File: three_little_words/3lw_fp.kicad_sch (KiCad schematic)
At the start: 19 parts, among them J10 Eurorack_Mono_Jack, J11 Eurorack_Mono_Jack, J12 Eurorack_Mono_Jack, J13 Eurorack_Mono_Jack, J14 Eurorack_Mono_Jack, J2 Eurorack_Mono_Jack, J3 Eurorack_Mono_Jack, J4 Eurorack_Mono_Jack, J5 Eurorack_Mono_Jack, J6 Eurorack_Mono_Jack, J7 Eurorack_Mono_Jack, J8 SSD1306_OLED_CONN, J9 Eurorack_Mono_Jack, SW1 SW_Push, SW2 SW_Push, SW3 SW_Push, SW4 RotaryEncoder_Switch, SW5 RotaryEncoder_Switch, SW6 RotaryEncoder_Switch

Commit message: Adding footprints for various components of 3lw.
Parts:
- J8: footprint (none) -> Connector_PinSocket_2.54mm:PinSocket_1x04_P2.54mm_Vertical
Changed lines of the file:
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@@
     (property "Reference" "J8" (id 0) (at 66.04 170.18 0))
     (property "Value" "SSD1306_OLED_CONN" (id 1) (at 66.04 172.72 0))
-    (property "Footprint" "" (id 2) (at 65.405 180.975 0)
+    (property "Footprint" "Connector_PinSocket_2.54mm:PinSocket_1x04_P2.54mm_Vertical" (id 2) (at 65.405 180.975 0)
       (effects (font (size 1.27 1.27)) hide)
     )

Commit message: Adding BOM, footprints, starting circuit.
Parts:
- J10, J11, J12, J13, J14, J2, J3, J4, J5, J6, J7, J9: footprint winterbloom:WQP-WQP518MA -> winterbloom:WQP518MA
- SW1, SW2, SW3: footprint (none) -> Button_Switch_THT:SW_PUSH_6mm
- SW4, SW5, SW6: footprint (none) -> Rotary_Encoder:RotaryEncoder_Alps_EC12E-Switch_Vertical_H20mm
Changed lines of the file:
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@@
     (property "Reference" "SW4" (id 0) (at 40.6938 111.506 0))
     (property "Value" "RotaryEncoder_Switch" (id 1) (at 40.6938 114.046 0))
-    (property "Footprint" "" (id 2) (at 36.8838 118.364 0)
+    (property "Footprint" "Rotary_Encoder:RotaryEncoder_Alps_EC12E-Switch_Vertical_H20mm" (id 2) (at 36.8838 118.364 0)
       (effects (font (size 1.27 1.27)) hide)
     )
@@
     (property "Reference" "J14" (id 0) (at 65.2048 108.458 0))
     (property "Value" "Eurorack_Mono_Jack" (id 1) (at 65.2048 105.918 0))
-    (property "Footprint" "winterbloom:WQP-WQP518MA" (id 2) (at 65.8398 106.553 0)
+    (property "Footprint" "winterbloom:WQP518MA" (id 2) (at 65.8398 106.553 0)
       (effects (font (size 1.27 1.27)) hide)
     )
@@
     (property "Reference" "SW3" (id 0) (at 40.4398 194.31 0))
     (property "Value" "SW_Push" (id 1) (at 40.4398 191.77 0))
-    (property "Footprint" "" (id 2) (at 40.4398 191.008 0)
+    (property "Footprint" "Button_Switch_THT:SW_PUSH_6mm" (id 2) (at 40.4398 191.008 0)
       (effects (font (size 1.27 1.27)) hide)
     )
@@
     (property "Reference" "J10" (id 0) (at 65.2048 44.958 0))
     (property "Value" "Eurorack_Mono_Jack" (id 1) (at 65.2048 42.418 0))
-    (property "Footprint" "winterbloom:WQP-WQP518MA" (id 2) (at 65.8398 43.053 0)
+    (property "Footprint" "winterbloom:WQP518MA" (id 2) (at 65.8398 43.053 0)
       (effects (font (size 1.27 1.27)) hide)
     )
@@
     (property "Reference" "J13" (id 0) (at 65.2048 92.583 0))
     (property "Value" "Eurorack_Mono_Jack" (id 1) (at 65.2048 90.043 0))
-    (property "Footprint" "winterbloom:WQP-WQP518MA" (id 2) (at 65.8398 90.678 0)
+    (property "Footprint" "winterbloom:WQP518MA" (id 2) (at 65.8398 90.678 0)
       (effects (font (size 1.27 1.27)) hide)
     )
@@
     (property "Reference" "J11" (id 0) (at 65.2048 60.833 0))
     (property "Value" "Eurorack_Mono_Jack" (id 1) (at 65.2048 58.293 0))
-    (property "Footprint" "winterbloom:WQP-WQP518MA" (id 2) (at 65.8398 58.928 0)
+    (property "Footprint" "winterbloom:WQP518MA" (id 2) (at 65.8398 58.928 0)
       (effects (font (size 1.27 1.27)) hide)
     )
@@
     (property "Reference" "J12" (id 0) (at 65.2048 76.708 0))
     (property "Value" "Eurorack_Mono_Jack" (id 1) (at 65.2048 74.168 0))
-    (property "Footprint" "winterbloom:WQP-WQP518MA" (id 2) (at 65.8398 74.803 0)
+    (property "Footprint" "winterbloom:WQP518MA" (id 2) (at 65.8398 74.803 0)
       (effects (font (size 1.27 1.27)) hide)
     )
@@
     (property "Reference" "J2" (id 0) (at 24.0568 15.113 0))
     (property "Value" "Eurorack_Mono_Jack" (id 1) (at 24.0568 17.653 0))
-    (property "Footprint" "winterbloom:WQP-WQP518MA" (id 2) (at 23.4218 17.018 0)
+    (property "Footprint" "winterbloom:WQP518MA" (id 2) (at 23.4218 17.018 0)
       (effects (font (size 1.27 1.27)) hide)
     )
@@
     (property "Reference" "SW2" (id 0) (at 40.386 184.15 0))
     (property "Value" "SW_Push" (id 1) (at 40.386 181.61 0))
-    (property "Footprint" "" (id 2) (at 40.386 180.848 0)
+    (property "Footprint" "Button_Switch_THT:SW_PUSH_6mm" (id 2) (at 40.386 180.848 0)
       (effects (font (size 1.27 1.27)) hide)
     )
@@
     (property "Reference" "SW1" (id 0) (at 40.386 173.99 0))
     (property "Value" "SW_Push" (id 1) (at 40.386 171.45 0))
-    (property "Footprint" "" (id 2) (at 40.386 170.688 0)
+    (property "Footprint" "Button_Switch_THT:SW_PUSH_6mm" (id 2) (at 40.386 170.688 0)
       (effects (font (size 1.27 1.27)) hide)
     )
@@
     (property "Reference" "J3" (id 0) (at 24.0568 30.988 0))
     (property "Value" "Eurorack_Mono_Jack" (id 1) (at 24.0568 33.528 0))
-    (property "Footprint" "winterbloom:WQP-WQP518MA" (id 2) (at 23.4218 32.893 0)
+    (property "Footprint" "winterbloom:WQP518MA" (id 2) (at 23.4218 32.893 0)
       (effects (font (size 1.27 1.27)) hide)
     )
@@
     (property "Reference" "J4" (id 0) (at 24.0568 46.863 0))
     (property "Value" "Eurorack_Mono_Jack" (id 1) (at 24.0568 49.403 0))
-    (property "Footprint" "winterbloom:WQP-WQP518MA" (id 2) (at 23.4218 48.768 0)
+    (property "Footprint" "winterbloom:WQP518MA" (id 2) (at 23.4218 48.768 0)
       (effects (font (size 1.27 1.27)) hide)
     )
@@
     (property "Reference" "J6" (id 0) (at 24.0568 78.613 0))
     (property "Value" "Eurorack_Mono_Jack" (id 1) (at 24.0568 81.153 0))
-    (property "Footprint" "winterbloom:WQP-WQP518MA" (id 2) (at 23.4218 80.518 0)
+    (property "Footprint" "winterbloom:WQP518MA" (id 2) (at 23.4218 80.518 0)
       (effects (font (size 1.27 1.27)) hide)
     )
@@
     (property "Reference" "J5" (id 0) (at 24.0568 62.738 0))
     (property "Value" "Eurorack_Mono_Jack" (id 1) (at 24.0568 65.278 0))
-    (property "Footprint" "winterbloom:WQP-WQP518MA" (id 2) (at 23.4218 64.643 0)
+    (property "Footprint" "winterbloom:WQP518MA" (id 2) (at 23.4218 64.643 0)
       (effects (font (size 1.27 1.27)) hide)
     )
@@
     (property "Reference" "SW5" (id 0) (at 40.6938 128.524 0))
     (property "Value" "RotaryEncoder_Switch" (id 1) (at 40.6938 131.064 0))
-    (property "Footprint" "" (id 2) (at 36.8838 135.382 0)
+    (property "Footprint" "Rotary_Encoder:RotaryEncoder_Alps_EC12E-Switch_Vertical_H20mm" (id 2) (at 36.8838 135.382 0)
       (effects (font (size 1.27 1.27)) hide)
     )
@@
     (property "Reference" "J7" (id 0) (at 24.0568 94.488 0))
     (property "Value" "Eurorack_Mono_Jack" (id 1) (at 24.0568 97.028 0))
-    (property "Footprint" "winterbloom:WQP-WQP518MA" (id 2) (at 23.4218 96.393 0)
+    (property "Footprint" "winterbloom:WQP518MA" (id 2) (at 23.4218 96.393 0)
       (effects (font (size 1.27 1.27)) hide)
     )
@@
     (property "Reference" "SW6" (id 0) (at 40.6938 145.542 0))
     (property "Value" "RotaryEncoder_Switch" (id 1) (at 40.6938 148.082 0))
-    (property "Footprint" "" (id 2) (at 36.8838 152.4 0)
+    (property "Footprint" "Rotary_Encoder:RotaryEncoder_Alps_EC12E-Switch_Vertical_H20mm" (id 2) (at 36.8838 152.4 0)
       (effects (font (size 1.27 1.27)) hide)
     )
@@
     (property "Reference" "J9" (id 0) (at 65.2048 29.083 0))
     (property "Value" "Eurorack_Mono_Jack" (id 1) (at 65.2048 26.543 0))
-    (property "Footprint" "winterbloom:WQP-WQP518MA" (id 2) (at 65.8398 27.178 0)
-      (effects (font (size 1.27 1.27)) hide)
-    )
+    (property "Footprint" "winterbloom:WQP518MA" (id 2) (at 65.8398 27.178 0)
+      (effects (font (size 1.27 1.27)) hide)
+    )

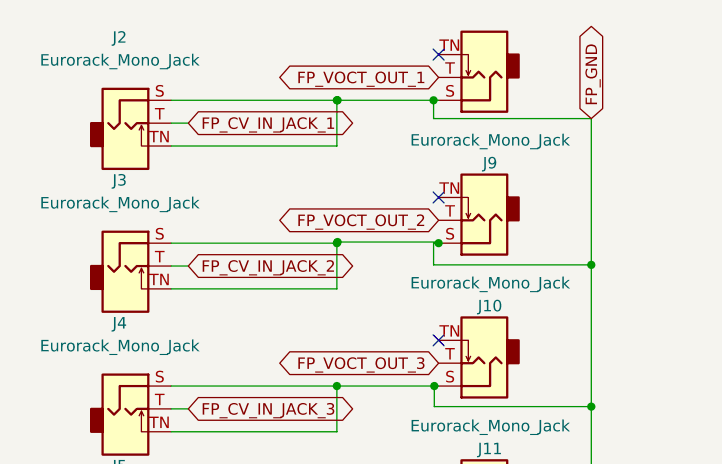
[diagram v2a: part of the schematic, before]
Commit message: Finishing 3lw schematic
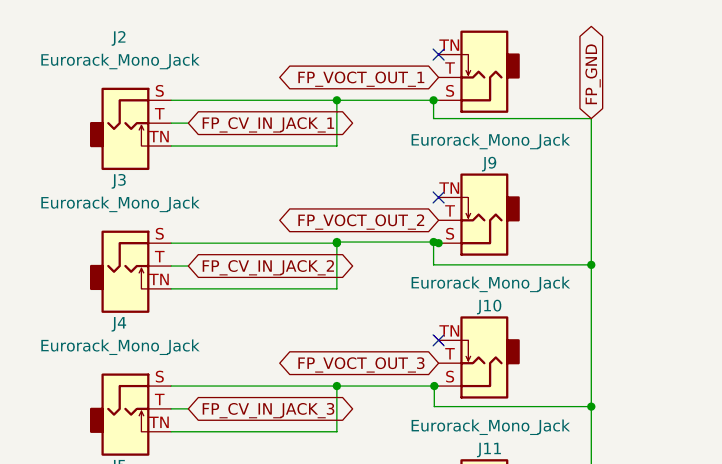
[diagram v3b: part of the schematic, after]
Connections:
- net FP_GND: now also J2.S (Sleeve), J2.TN (Tip_normalize), J3.S (Sleeve), J3.TN (Tip_normalize)
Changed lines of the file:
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@@
   (junction (at 50.0918 101.473) (diameter 0) (color 0 0 0 0)
   )
+  (junction (at 48.1868 37.973) (diameter 0) (color 0 0 0 0)
+  )
+  (junction (at 59.4898 37.973) (diameter 0) (color 0 0 0 0)
+  )
   (junction (at 58.8548 101.473) (diameter 0) (color 0 0 0 0)
   )
+  (junction (at 58.928 22.098) (diameter 0) (color 0 0 0 0)
+  )
+  (junction (at 52.9685 141.986) (diameter 0) (color 0 0 0 0)
+  )
+  (junction (at 76.454 103.886) (diameter 0) (color 0 0 0 0)
+  )
+  (junction (at 76.454 40.386) (diameter 0) (color 0 0 0 0)
+  )
+  (junction (at 48.4313 162.814) (diameter 0) (color 0 0 0 0)
+  )
+  (junction (at 52.3879 159.004) (diameter 0) (color 0 0 0 0)
+  )
+  (junction (at 48.1868 53.848) (diameter 0) (color 0 0 0 0)
+  )
+  (junction (at 58.928 37.846) (diameter 0) (color 0 0 0 0)
+  )
+  (junction (at 59.01 53.848) (diameter 0) (color 0 0 0 0)
+  )
+  (junction (at 76.454 141.986) (diameter 0) (color 0 0 0 0)
+  )
+  (junction (at 76.454 71.882) (diameter 0) (color 0 0 0 0)
+  )
+  (junction (at 50.0918 69.723) (diameter 0) (color 0 0 0 0)
+  )
+  (junction (at 58.8847 85.598) (diameter 0) (color 0 0 0 0)
+  )
   (junction (at 48.1868 22.098) (diameter 0) (color 0 0 0 0)
   )
-  (junction (at 48.1868 37.973) (diameter 0) (color 0 0 0 0)
-  )
-  (junction (at 52.9685 141.986) (diameter 0) (color 0 0 0 0)
-  )
-  (junction (at 48.26 37.846) (diameter 0) (color 0 0 0 0)
-  )
-  (junction (at 76.454 103.886) (diameter 0) (color 0 0 0 0)
-  )
-  (junction (at 76.454 40.386) (diameter 0) (color 0 0 0 0)
-  )
-  (junction (at 48.4313 162.814) (diameter 0) (color 0 0 0 0)
-  )
-  (junction (at 52.3879 159.004) (diameter 0) (color 0 0 0 0)
-  )
-  (junction (at 48.1868 53.848) (diameter 0) (color 0 0 0 0)
-  )
-  (junction (at 59.01 53.848) (diameter 0) (color 0 0 0 0)
-  )
-  (junction (at 76.454 141.986) (diameter 0) (color 0 0 0 0)
-  )
-  (junction (at 58.928 22.098) (diameter 0) (color 0 0 0 0)
-  )
-  (junction (at 76.454 71.882) (diameter 0) (color 0 0 0 0)
-  )
-  (junction (at 50.0918 69.723) (diameter 0) (color 0 0 0 0)
-  )
-  (junction (at 58.8847 85.598) (diameter 0) (color 0 0 0 0)
-  )
   (junction (at 52.6202 124.968) (diameter 0) (color 0 0 0 0)
   )
@@
   (junction (at 76.454 87.884) (diameter 0) (color 0 0 0 0)
   )
-  (junction (at 59.4898 37.973) (diameter 0) (color 0 0 0 0)
-  )
-  (junction (at 48.26 22.098) (diameter 0) (color 0 0 0 0)
-  )
   (junction (at 76.454 124.968) (diameter 0) (color 0 0 0 0)
+  )
+  (junction (at 48.1868 37.846) (diameter 0) (color 0 0 0 0)
   )
   (no_connect (at 59.4898 48.768))
@@
     (stroke (width 0) (type default) (color 0 0 0 0))
   )
+  (wire (pts (xy 59.4898 37.973) (xy 59.4898 37.846))
+    (stroke (width 0) (type default) (color 0 0 0 0))
+  )
   (wire (pts (xy 48.3138 159.004) (xy 52.3879 159.004))
     (stroke (width 0) (type default) (color 0 0 0 0))
   )
-  (wire (pts (xy 58.928 37.973) (xy 59.4898 37.973))
-    (stroke (width 0) (type default) (color 0 0 0 0))
-  )
   (wire (pts (xy 48.1868 53.848) (xy 59.01 53.848))
     (stroke (width 0) (type default) (color 0 0 0 0))
@@
     (stroke (width 0) (type default) (color 0 0 0 0))
   )
+  (wire (pts (xy 48.1868 37.846) (xy 48.1868 37.973))
+    (stroke (width 0) (type default) (color 0 0 0 0))
+  )
   (wire (pts (xy 29.7718 37.973) (xy 48.1868 37.973))
     (stroke (width 0) (type default) (color 0 0 0 0))
@@
     (stroke (width 0) (type default) (color 0 0 0 0))
   )
-  (wire (pts (xy 59.4898 37.846) (xy 59.4898 37.973))
-    (stroke (width 0) (type default) (color 0 0 0 0))
-  )
   (wire (pts (xy 70.485 180.975) (xy 71.755 180.975))
     (stroke (width 0) (type default) (color 0 0 0 0))
@@
     (stroke (width 0) (type default) (color 0 0 0 0))
   )
-  (wire (pts (xy 58.928 40.386) (xy 58.928 37.973))
+  (wire (pts (xy 58.928 37.846) (xy 58.928 40.386))
     (stroke (width 0) (type default) (color 0 0 0 0))
   )
@@
     (stroke (width 0) (type default) (color 0 0 0 0))
   )
-  (wire (pts (xy 48.26 22.098) (xy 58.928 22.098))
-    (stroke (width 0) (type default) (color 0 0 0 0))
-  )
   (wire (pts (xy 52.6202 124.968) (xy 76.454 124.968))
     (stroke (width 0) (type default) (color 0 0 0 0))
@@
     (stroke (width 0) (type default) (color 0 0 0 0))
   )
+  (wire (pts (xy 59.4898 37.846) (xy 58.928 37.846))
+    (stroke (width 0) (type default) (color 0 0 0 0))
+  )
   (wire (pts (xy 45.466 175.768) (xy 45.466 185.928))
     (stroke (width 0) (type default) (color 0 0 0 0))
@@
     (stroke (width 0) (type default) (color 0 0 0 0))
   )
-  (wire (pts (xy 48.26 37.846) (xy 59.4898 37.846))
-    (stroke (width 0) (type default) (color 0 0 0 0))
-  )
   (wire (pts (xy 29.7718 27.178) (xy 48.1868 27.178))
     (stroke (width 0) (type default) (color 0 0 0 0))
@@
     (stroke (width 0) (type default) (color 0 0 0 0))
   )
+  (wire (pts (xy 48.1868 22.098) (xy 58.928 22.098))
+    (stroke (width 0) (type default) (color 0 0 0 0))
+  )
   (wire (pts (xy 50.0918 69.723) (xy 58.9573 69.723))
     (stroke (width 0) (type default) (color 0 0 0 0))
   )
+  (wire (pts (xy 58.928 37.846) (xy 48.1868 37.846))
+    (stroke (width 0) (type default) (color 0 0 0 0))
+  )
